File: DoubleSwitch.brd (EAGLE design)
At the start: 27.5 x 46.9 mm, 36 parts, among them IC1 LNK304, IC3 MC33269ST-3.3T3, K1 FRS1B, K2 FRS1B, T1 BC846, T2 BC846, X1 16 MHz

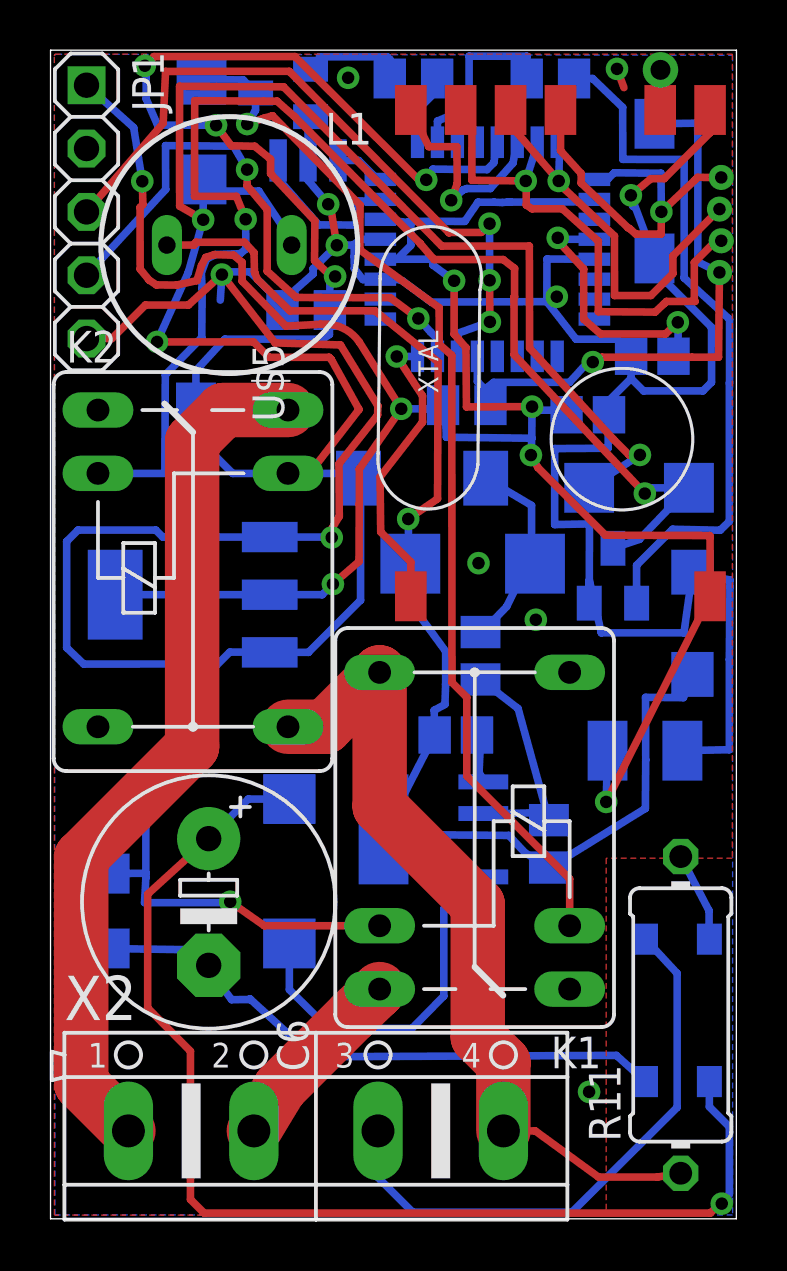
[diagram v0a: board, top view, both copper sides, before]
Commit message: aaa
aaa
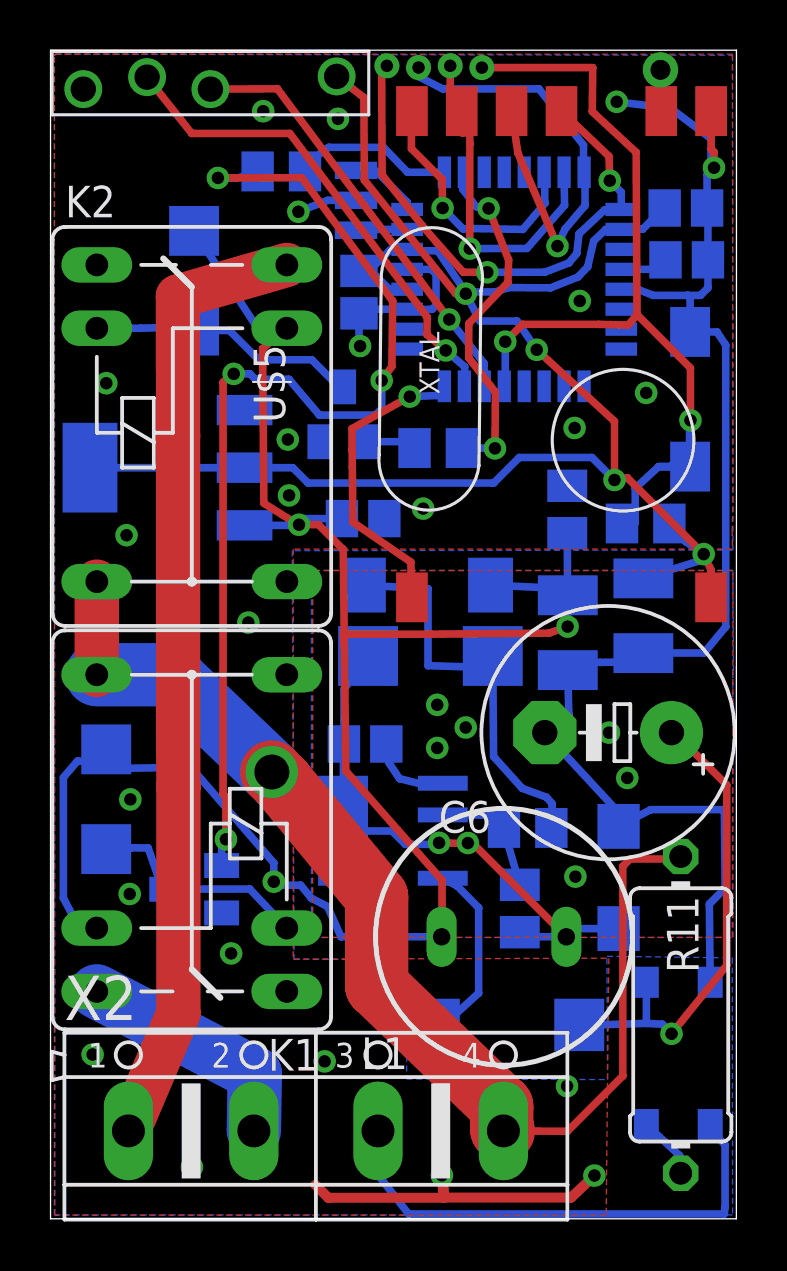
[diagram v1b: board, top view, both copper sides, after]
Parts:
- removed R14: 560, resistor:M2012
- added C2, C3: 0.1, resistor:C2012
- JP1: value (none) -> PINHD1X5SQUARE; device pinhead-2:1X05-S -> eagle-library-edeca.net-v5:PINHD1X05-SQUARE
- R4: value 560 -> 1K
- moved T1 32.1 mm to (5.76, 13.2)
- moved L1 29.8 mm to (18.2, 11.3), turned to 180 degrees
- moved D1 27.1 mm to (2.24, 16.8), turned to 270 degrees
- moved C11 21.8 mm to (20.7, 23.5)
- moved D2 19.7 mm to (5.76, 37.6), turned to 270 degrees
- moved C6 17.4 mm to (22.4, 19.5), turned to 180 degrees
- moved R3 15.5 mm to (15.5, 30.9), turned to 0 degrees
- moved R4 15.3 mm to (20.7, 28.4)
- moved U$2 12.9 mm to (16.0, 46.2), turned to 180 degrees
- moved T2 12.6 mm to (11.8, 32.3)
- moved K1 11.3 mm to (5.66, 11.7)
- moved R10 10.7 mm to (18.3, 7.78), turned to 0 degrees
- moved D3 10.6 mm to (22.8, 13.7)
- moved C10 9.18 mm to (25.5, 40.5)
- moved R1 8.60 mm to (23.9, 27.9), turned to 0 degrees
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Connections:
- net N$10 renamed S
- removed net N$8: K1.P, K2.P, R11.1, X2.4
- net 5V: now also C2.1
- net D9: no longer R14.2, R4.1
- net GND: now also C2.2, C3.2, R4.1; no longer R14.1
- net N$16: now also K1.P, R11.1, X2.4
- net VCC: now also C3.1
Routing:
- net GND: track 153.6 -> 81.1 mm, vias 11 -> 24
- net N$16: track 0.00 -> 47.0 mm, vias 0 -> 1
- net N$4: track 53.9 -> 12.0 mm, vias 2 -> 0
- net D9: track 40.7 -> 0.07 mm, vias 4 -> 0
- net N$2: track 5.13 -> 42.5 mm, vias 0 -> 4
- net N$5: track 42.5 -> 9.08 mm, vias 1 -> 0
- net N$8: track 32.7 -> 0.00 mm
- net S: track 53.5 -> 23.5 mm, vias 1 -> 8
- net N$14: track 47.6 -> 19.3 mm
- net N$6: track 28.3 -> 2.15 mm
- net VCC: track 95.2 -> 72.4 mm, vias 7 -> 4
- net 5V: track 102.3 -> 82.3 mm, vias 4 -> 3
- net D0_RX: track 28.9 -> 17.4 mm, vias 3 -> 1
- net RST: track 24.6 -> 34.9 mm, vias 1 -> 2
- net AREF: track 10.8 -> 1.93 mm, vias 2 -> 0
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- added copper zone on layer 1, net S
- added copper zone on layer 16, net S
